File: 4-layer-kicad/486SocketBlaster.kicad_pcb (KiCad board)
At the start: 4 copper layers, 47.6 x 51.8 mm, 20 parts, among them U1 TPS563200

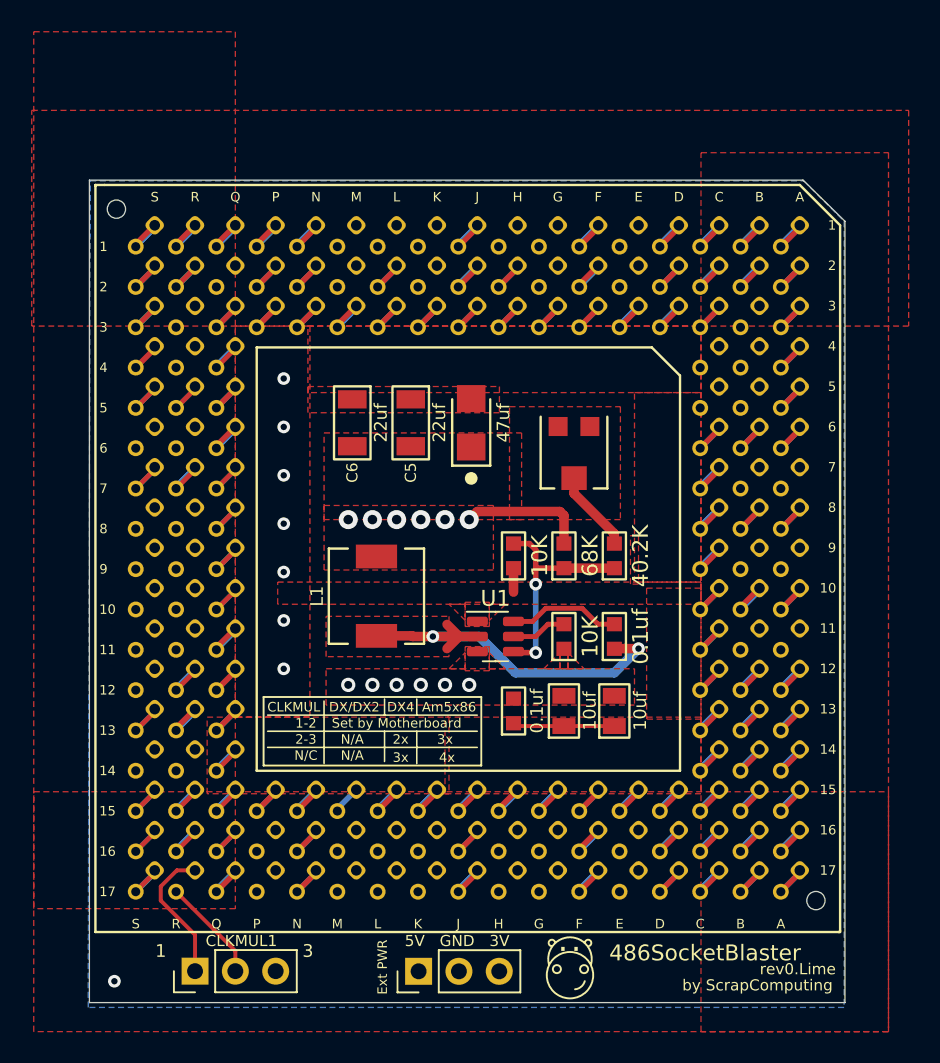
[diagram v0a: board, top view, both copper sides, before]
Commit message: update
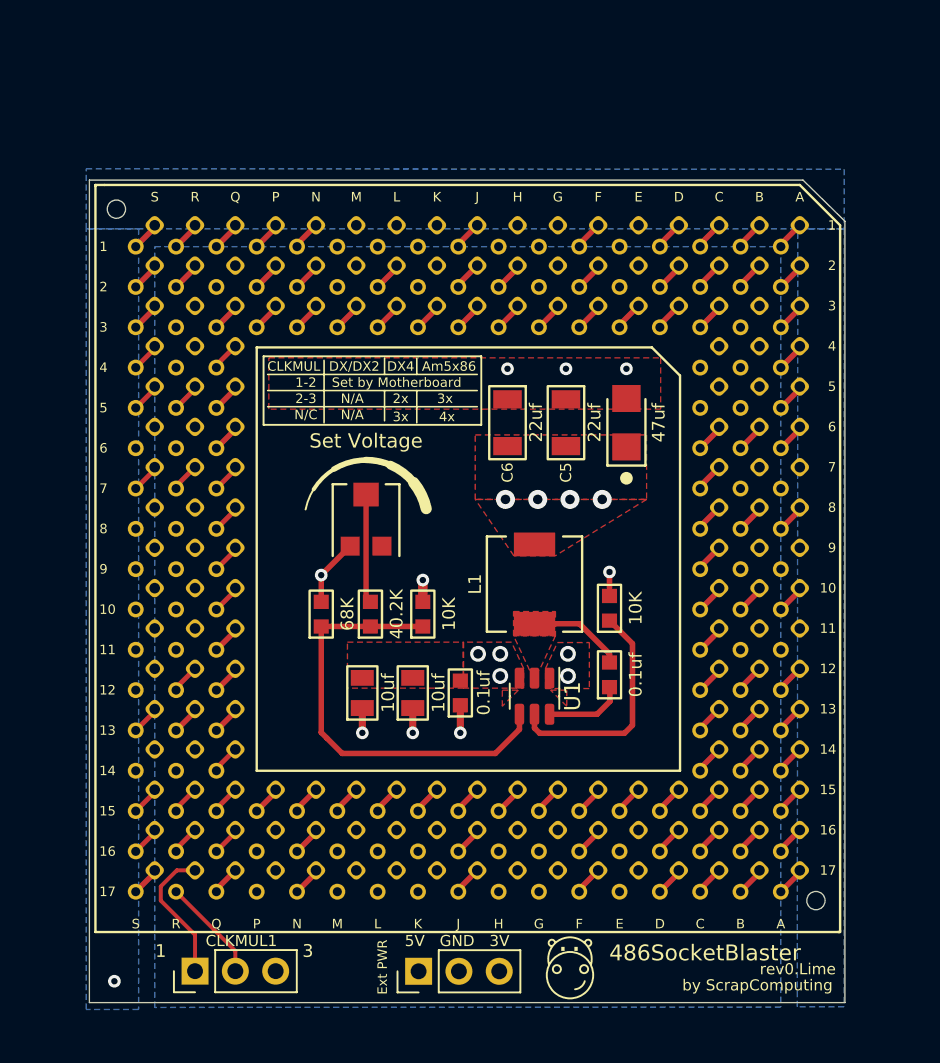
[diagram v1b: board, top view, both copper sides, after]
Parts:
- moved R4 15.8 mm to (115.2, 56.2)
- moved R2 15.7 mm to (112.1, 56.2)
- moved RV1 13.7 mm to (114.9, 50.2), turned to -90 degrees
- moved C2 12.8 mm to (117.9, 61.2)
- moved C1 12.8 mm to (114.7, 61.2)
- moved L1 9.99 mm to (125.5, 54.4)
- moved C7 9.78 mm to (131.3, 44.2)
- moved C5 9.78 mm to (127.5, 44.2)
- moved C6 9.78 mm to (123.8, 44.2)
- moved R3 6.79 mm to (118.5, 56.2)
- moved U1 4.49 mm to (125.5, 61.4), turned to -90 degrees
- moved C3 3.54 mm to (120.9, 61.2)
- moved R1 3.38 mm to (130.3, 55.9)
- moved C4 2.43 mm to (130.3, 60.1)
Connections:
- net Net-(RV1-Pad2) renamed /Trim
- C4 pad 1: SW -> Net-(U1-Pad6)
- C4 pad 2: Net-(C4-Pad2) -> /SW
- L1 pad 1: SW -> /SW
- R1 pad 1: Vin -> Net-(U1-Pad5)
- R1 pad 2: Net-(R1-Pad2) -> Vin
- R2 pad 1: FBVoltage -> /FBVoltage
- R3 pad 1: GND -> /FBVoltage
- R3 pad 2: FBVoltage -> GND
- R4 pad 1: FBVoltage -> /FBVoltage
- RV1 pad 1: Vout -> unconnected-(RV1-Pad1)
- RV1 pad 3: unconnected-(RV1-Pad3) -> Vout
- U1 pad 2: SW -> /SW
- U1 pad 4: FBVoltage -> /FBVoltage
- U1 pad 5: Net-(R1-Pad2) -> Net-(U1-Pad5)
- U1 pad 6: Net-(C4-Pad2) -> Net-(U1-Pad6)
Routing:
- net /FBVoltage: track 0.00 -> 28.0 mm
- net SW: track 24.6 -> 0.00 mm, vias 2 -> 0
- net Net-(U1-Pad5): track 0.00 -> 14.6 mm
- net FBVoltage: track 14.3 -> 0.00 mm, vias 2 -> 0
- net Net-(C4-Pad2): track 7.11 -> 0.00 mm
- net /SW: track 0.00 -> 6.05 mm
- net Net-(U1-Pad6): track 0.00 -> 5.04 mm
- net Vout: track 8.05 -> 4.26 mm, vias 6 -> 5
- net Net-(R1-Pad2): track 3.50 -> 0.00 mm
- net GND: track 8.60 -> 6.39 mm, vias 8 -> 10
- net Net-(Pins1-PadE3): track 3.68 -> 1.84 mm
- net Net-(Pins1-PadQ16): track 3.68 -> 1.84 mm
- net Net-(Pins1-PadQ14): track 3.53 -> 1.69 mm
- net Net-(Pins1-PadN16): track 3.68 -> 1.84 mm
- net Net-(Pins1-PadE15): track 3.68 -> 1.84 mm
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- added copper zone on F.Cu, net /SW
- added copper zone on B.Cu, net Vout
- removed copper zone on F.Cu, net SW
- removed copper zone on In1.Cu, net Vout
